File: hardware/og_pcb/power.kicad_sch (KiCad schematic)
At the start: 4 parts, among them J3 Barrel_Jack, U4 BD33FC0FP

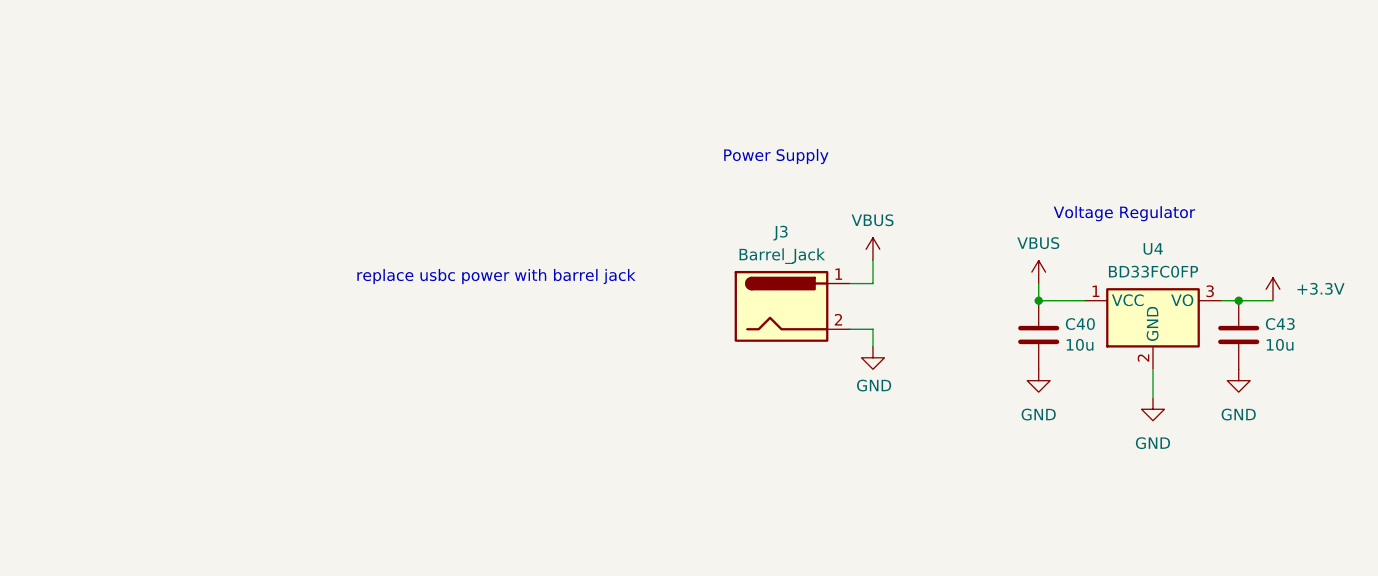
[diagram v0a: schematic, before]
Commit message: new preliminary demo pcb
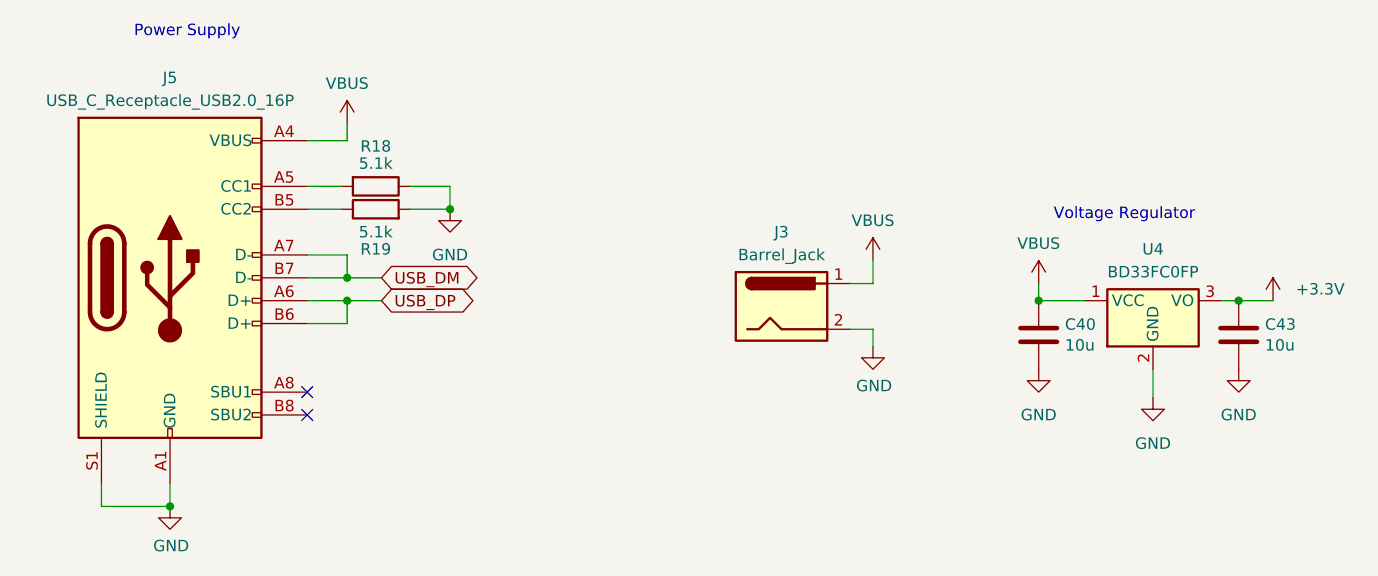
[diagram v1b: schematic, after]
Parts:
- added J5: USB_C_Receptacle_USB2.0_16P, 1my_footprints:microUSB, symbol Connector:USB_C_Receptacle_USB2.0_16P
- added R18, R19: 5.1k, Resistor_SMD:R_0402_1005Metric, symbol Device:R
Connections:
- net GND: now also J5.A1 (GND), J5.A12 (GND), J5.B1 (GND), J5.B12 (GND), J5.S1 (SHIELD), R18.1, R19.2
- net VBUS: now also J5.A4 (VBUS), J5.A9 (VBUS), J5.B4 (VBUS), J5.B9 (VBUS)
- new net: J5.A5 (CC1), R18.2
- new net: J5.B5 (CC2), R19.1
- new net USB_DM: J5.A7 (D-), J5.B7 (D-)
- new net USB_DP: J5.A6 (D+), J5.B6 (D+)
- no-connect marks 0 -> 2
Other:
- note removed: "replace usbc power with barrel jack"
